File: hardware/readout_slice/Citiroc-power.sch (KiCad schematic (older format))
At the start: 2 parts

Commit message: need to fix one rescure in readout_slice
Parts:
- U? (x2): symbol readout_slice-rescue:CITIROC1A-readout -> readout_slice-rescue:CITIROC1A-readout-readout_slice-rescue
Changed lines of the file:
@@
 $Descr A4 11693 8268
 encoding utf-8
-Sheet 4 16
+Sheet 14 16
 Title ""
 Date ""
@@
 AR Path="/608039EA/60807685" Ref="#PWR?"  Part="1"
 AR Path="/6086954E/60943779/60807685" Ref="#PWR?"  Part="1"
+AR Path="/607ECAFE/60807685" Ref="#PWR?"  Part="1"
 F 0 "#PWR?" H 4000 6050 50  0001 C CNN
 F 1 "+5V" H 4000 6350 50  0000 C CNB
@@
 AR Path="/608039EA/60807697" Ref="#PWR?"  Part="1"
 AR Path="/6086954E/60943779/60807697" Ref="#PWR?"  Part="1"
+AR Path="/607ECAFE/60807697" Ref="#PWR?"  Part="1"
 F 0 "#PWR?" H 3850 1850 50  0001 C CNN
 F 1 "+3.3V" H 3850 2150 50  0000 C CNB
@@
 AR Path="/608039EA/608076AA" Ref="#PWR?"  Part="1"
 AR Path="/6086954E/60943779/608076AA" Ref="#PWR?"  Part="1"
+AR Path="/607ECAFE/608076AA" Ref="#PWR?"  Part="1"
 F 0 "#PWR?" H 2350 6150 50  0001 C CNN
 F 1 "GNDA" H 2350 6250 50  0000 C CNB
@@
 AR Path="/608039EA/608076B0" Ref="#PWR?"  Part="1"
 AR Path="/6086954E/60943779/608076B0" Ref="#PWR?"  Part="1"
+AR Path="/607ECAFE/608076B0" Ref="#PWR?"  Part="1"
 F 0 "#PWR?" H 2100 6150 50  0001 C CNN
 F 1 "GNDD" H 2100 6250 50  0000 C CNB
@@
 	2350 2400 2450 2400
 $Comp
-L readout_slice-rescue:CITIROC1A-readout U?
+L readout_slice-rescue:CITIROC1A-readout-readout_slice-rescue U?
 U 1 1 608076C8
 P 3650 4150
@@
 AR Path="/608039EA/608076C8" Ref="U?"  Part="1"
 AR Path="/6086954E/60943779/608076C8" Ref="U?"  Part="1"
+AR Path="/607ECAFE/608076C8" Ref="U?"  Part="1"
 F 0 "U?" V 1350 3800 50  0000 L CNN
 F 1 "CITIROC1A" V 1450 3800 50  0000 L CNN
@@
 AR Path="/608039EA/611876D0" Ref="#PWR?"  Part="1"
 AR Path="/6086954E/60943779/611876D0" Ref="#PWR?"  Part="1"
+AR Path="/607ECAFE/611876D0" Ref="#PWR?"  Part="1"
 F 0 "#PWR?" H 8500 5450 50  0001 C CNN
 F 1 "+5V" H 8500 5750 50  0000 C CNB
@@
 AR Path="/608039EA/611876E2" Ref="#PWR?"  Part="1"
 AR Path="/6086954E/60943779/611876E2" Ref="#PWR?"  Part="1"
+AR Path="/607ECAFE/611876E2" Ref="#PWR?"  Part="1"
 F 0 "#PWR?" H 8350 1250 50  0001 C CNN
 F 1 "+3.3V" H 8350 1550 50  0000 C CNB
@@
 AR Path="/608039EA/611876F5" Ref="#PWR?"  Part="1"
 AR Path="/6086954E/60943779/611876F5" Ref="#PWR?"  Part="1"
+AR Path="/607ECAFE/611876F5" Ref="#PWR?"  Part="1"
 F 0 "#PWR?" H 6850 5550 50  0001 C CNN
 F 1 "GNDA" H 6850 5650 50  0000 C CNB
@@
 AR Path="/608039EA/611876FB" Ref="#PWR?"  Part="1"
 AR Path="/6086954E/60943779/611876FB" Ref="#PWR?"  Part="1"
+AR Path="/607ECAFE/611876FB" Ref="#PWR?"  Part="1"
 F 0 "#PWR?" H 6600 5550 50  0001 C CNN
 F 1 "GNDD" H 6600 5650 50  0000 C CNB
@@
 	6850 1800 6950 1800
 $Comp
-L readout_slice-rescue:CITIROC1A-readout U?
+L readout_slice-rescue:CITIROC1A-readout-readout_slice-rescue U?
 U 1 1 61187713
 P 8150 3550
@@
 AR Path="/608039EA/61187713" Ref="U?"  Part="1"
 AR Path="/6086954E/60943779/61187713" Ref="U?"  Part="1"
+AR Path="/607ECAFE/61187713" Ref="U?"  Part="1"
 F 0 "U?" V 5850 3200 50  0000 L CNN
 F 1 "CITIROC1A" V 5950 3200 50  0000 L CNN

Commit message: getting rid of readout_slice rescue
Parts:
- U? (x2): symbol readout_slice-rescue:CITIROC1A-readout-readout_slice-rescue -> readout:CITIROC1A
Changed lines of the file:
@@
 	2350 2400 2450 2400
 $Comp
-L readout_slice-rescue:CITIROC1A-readout-readout_slice-rescue U?
+L readout:CITIROC1A U?
 U 1 1 608076C8
 P 3650 4150
@@
 	6850 1800 6950 1800
 $Comp
-L readout_slice-rescue:CITIROC1A-readout-readout_slice-rescue U?
+L readout:CITIROC1A U?
 U 1 1 61187713
 P 8150 3550

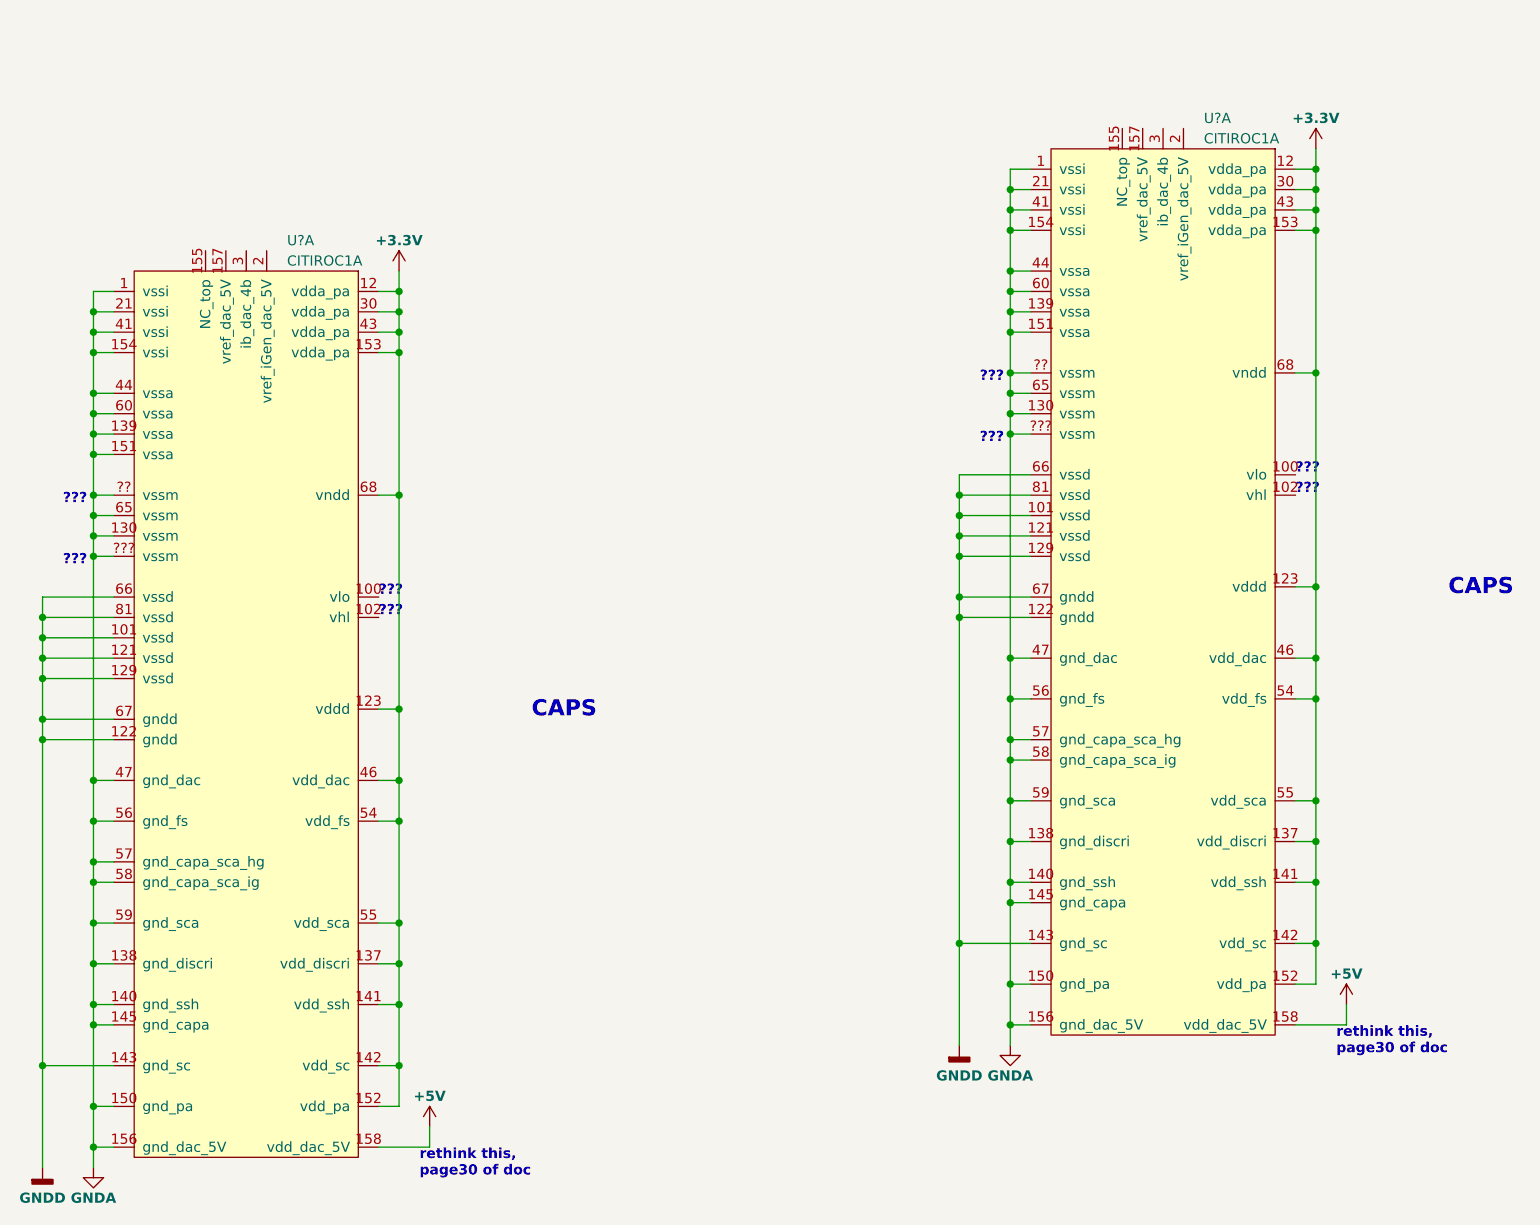
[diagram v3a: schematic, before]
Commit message: more progress on readout_slice
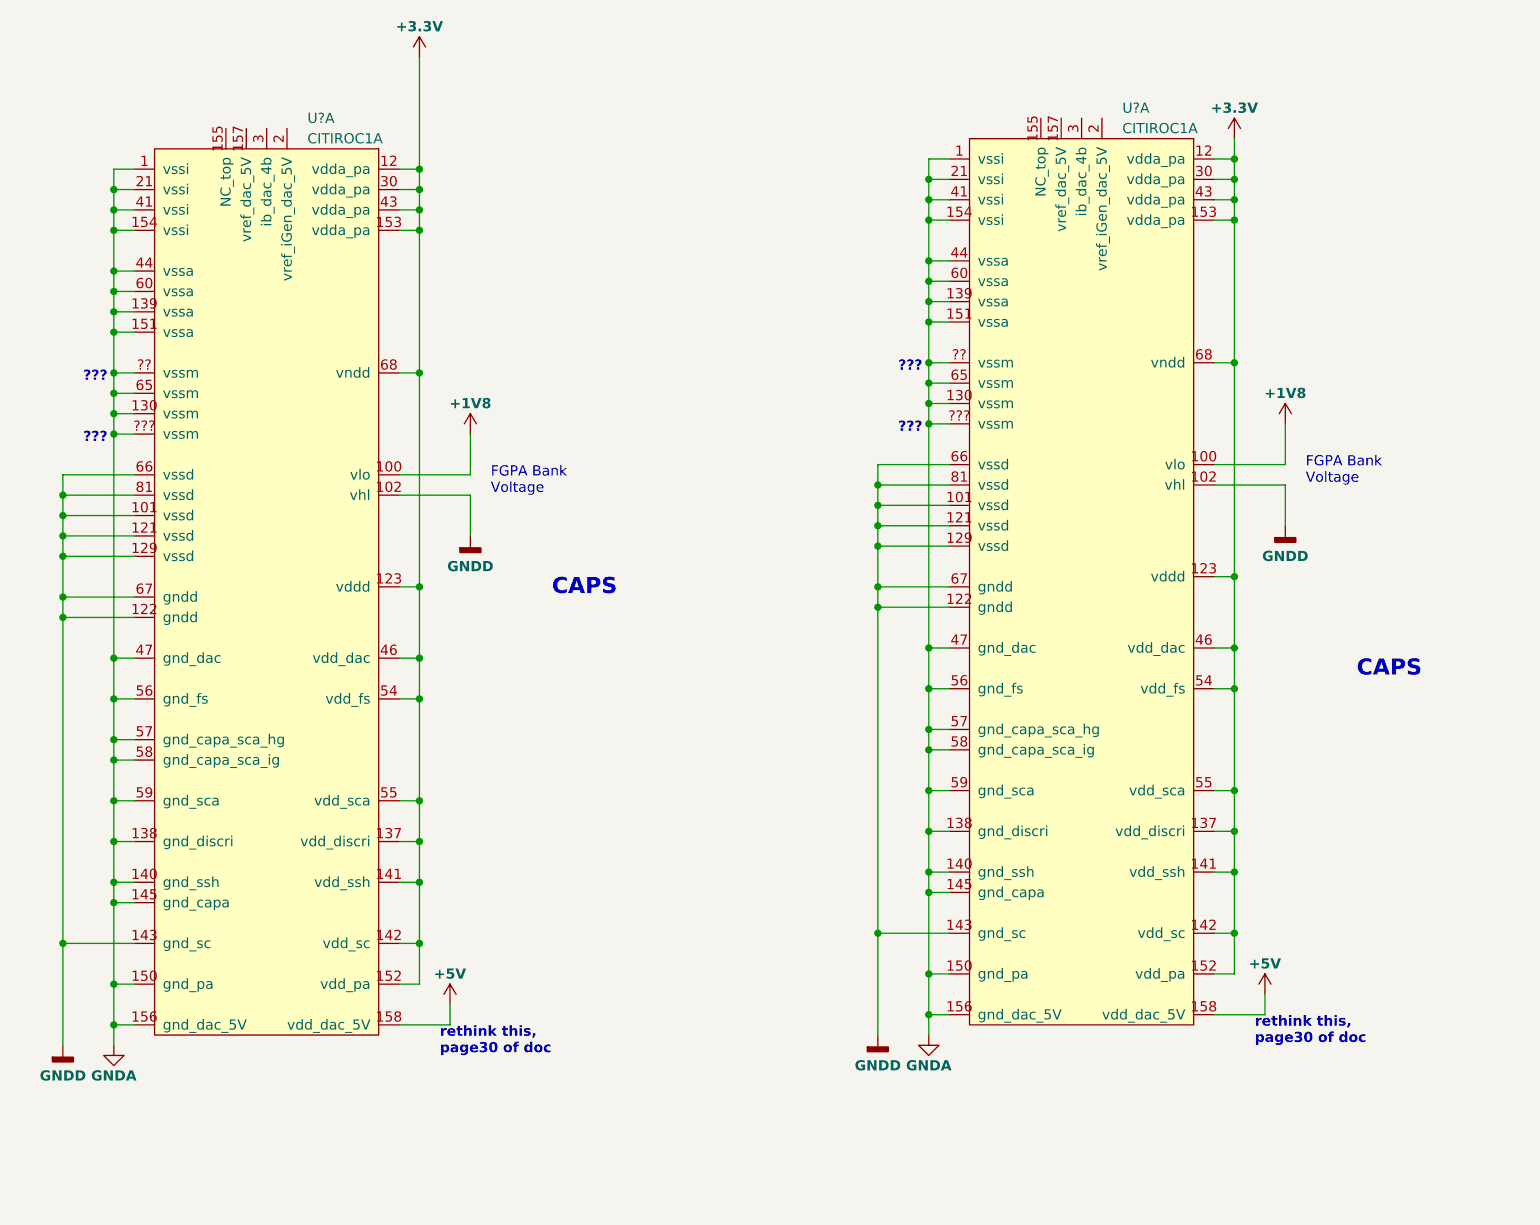
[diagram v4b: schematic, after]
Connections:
- net GNDD: now also U?.102 (vhl), U?.102 (vhl)
- net +1V8: now reaches U?.100 (vlo)
- net +1V8: now also U?.100 (vlo)
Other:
- note added: "FGPA Bank\nVoltage"
- moved on the sheet: U?A
